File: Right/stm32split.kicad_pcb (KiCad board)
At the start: 2 copper layers, 152.5 x 110.2 mm, 88 parts, among them J1 Conn_01x04, SW1 SW_Push, SW10 SW_Push, SW11 SW_Push, SW12 SW_Push, SW13 SW_Push, SW14 SW_Push, SW15 SW_Push, SW16 SW_Push, SW17 SW_Push, SW18 SW_Push, SW19 SW_Push, SW2 SW_Push, SW20 SW_Push, SW21 SW_Push, SW22 SW_Push, SW23 SW_Push, SW24 SW_Push, SW25 SW_Push, SW26 SW_Push, SW27 SW_Push, SW28 SW_Push, SW29 SW_Push, SW3 SW_Push, SW30 SW_Push, SW31 SW_Push, SW4 SW_Push, SW5 SW_Push, SW6 SW_Push, SW7 SW_Push, SW8 SW_Push, SW9 SW_Push, U1 SRV05-4, U2 STM32F103CBTx, U3 XC6206PxxxMR, Y1 8MHz

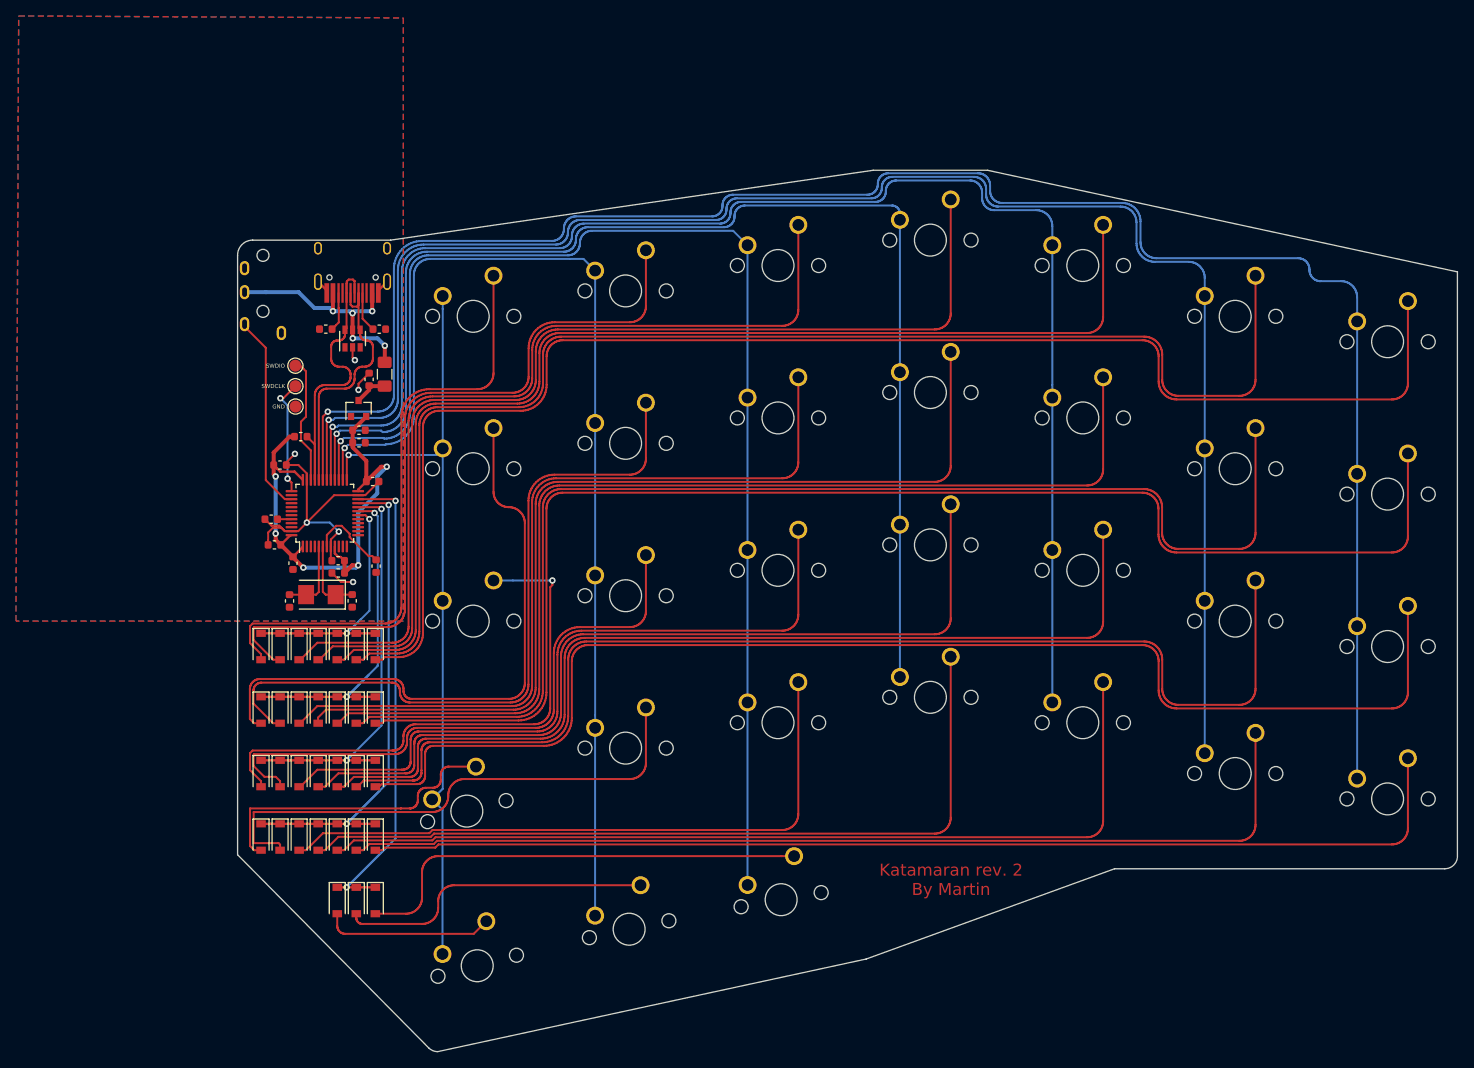
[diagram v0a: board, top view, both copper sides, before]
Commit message: rev2
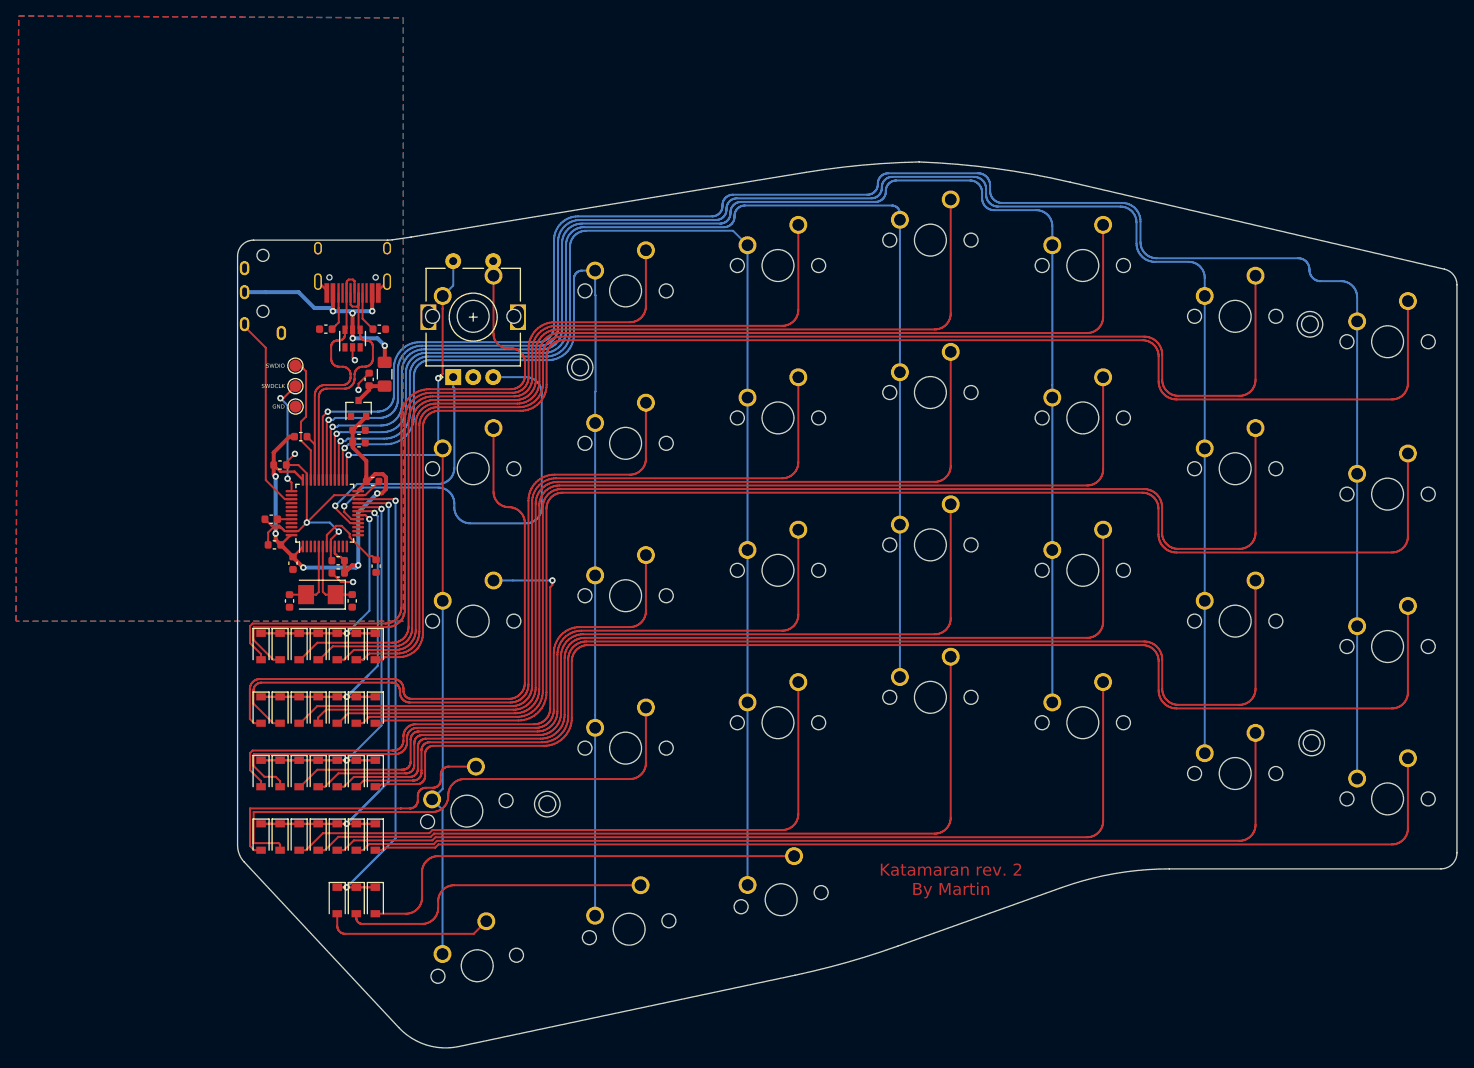
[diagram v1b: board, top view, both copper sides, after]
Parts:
- added REF**: MountingHole_3.2mm_M3, MountingHole:MountingHole_3.2mm_M3, F.Cu at (134.9, 67.3)
- added REF**: MountingHole_3.2mm_M3, MountingHole:MountingHole_3.2mm_M3, F.Cu at (226.1, 61.9)
- added REF**: MountingHole_3.2mm_M3, MountingHole:MountingHole_3.2mm_M3, F.Cu at (226.3, 114.3)
- added REF**: MountingHole_3.2mm_M3, MountingHole:MountingHole_3.2mm_M3, F.Cu at (130.8, 121.9)
- added REF**: RotaryEncoder_Alps_EC11E-Switch_Vertical_H20mm, Rotary_Encoder:RotaryEncoder_Alps_EC11E-Switch_Vertical_H20mm, F.Cu at (119.0, 68.5)
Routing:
- net Net-(U2-Pad17): track 0.00 -> 53.9 mm, vias 0 -> 1
- net Net-(U2-Pad16): track 0.00 -> 32.5 mm, vias 0 -> 1
- net Net-(D7-Pad2): track 75.6 -> 83.9 mm
- net COL6: track 98.6 -> 104.0 mm, vias 1 -> 2
- net COL5: track 137.6 -> 133.8 mm
- net VBAT: track 68.8 -> 67.7 mm
- net COL3: track 158.6 -> 157.6 mm
- net COL4: track 159.0 -> 158.1 mm
- net COL2: track 184.6 -> 183.8 mm
- net COL1: track 209.5 -> 208.7 mm
- net COL0: track 232.0 -> 231.2 mm
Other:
- board size 152.5 x 110.2 mm -> 152.4 x 110.7 mm
